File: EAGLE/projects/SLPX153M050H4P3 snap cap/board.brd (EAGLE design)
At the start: 139.7 x 64.4 mm, 6 parts

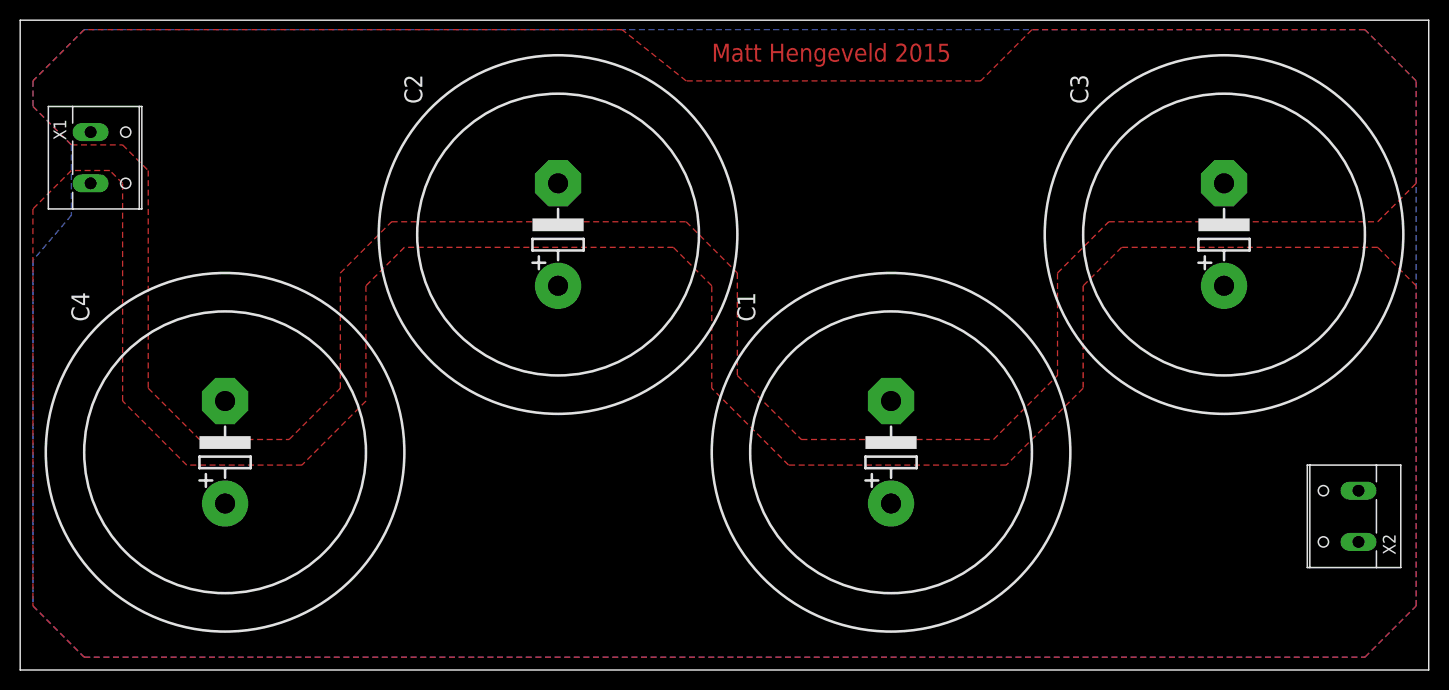
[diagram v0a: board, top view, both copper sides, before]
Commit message: a lot
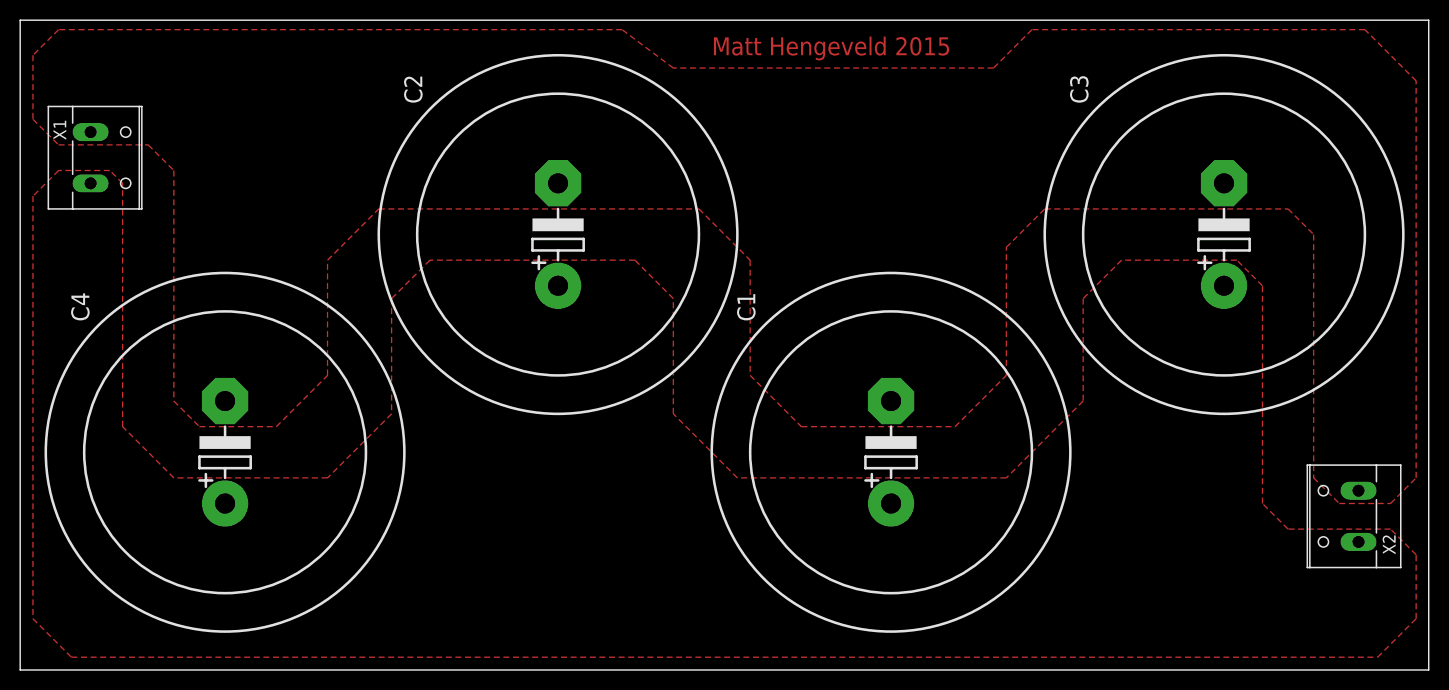
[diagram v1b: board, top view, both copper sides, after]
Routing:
- removed copper zone on layer 16, net GND
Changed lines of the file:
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@@
 <layer number="14" name="Route14" color="1" fill="6" visible="no" active="no"/>
 <layer number="15" name="Route15" color="4" fill="6" visible="no" active="no"/>
-<layer number="16" name="Bottom" color="1" fill="1" visible="yes" active="yes"/>
-<layer number="17" name="Pads" color="2" fill="1" visible="yes" active="yes"/>
-<layer number="18" name="Vias" color="2" fill="1" visible="yes" active="yes"/>
-<layer number="19" name="Unrouted" color="6" fill="1" visible="yes" active="yes"/>
-<layer number="20" name="Dimension" color="15" fill="1" visible="yes" active="yes"/>
-<layer number="21" name="tPlace" color="7" fill="1" visible="yes" active="yes"/>
-<layer number="22" name="bPlace" color="7" fill="1" visible="yes" active="yes"/>
-<layer number="23" name="tOrigins" color="15" fill="1" visible="yes" active="yes"/>
-<layer number="24" name="bOrigins" color="15" fill="1" visible="yes" active="yes"/>
-<layer number="25" name="tNames" color="7" fill="1" visible="yes" active="yes"/>
-<layer number="26" name="bNames" color="7" fill="1" visible="yes" active="yes"/>
-<layer number="27" name="tValues" color="7" fill="1" visible="yes" active="yes"/>
-<layer number="28" name="bValues" color="7" fill="1" visible="yes" active="yes"/>
+<layer number="16" name="Bottom" color="1" fill="1" visible="no" active="yes"/>
+<layer number="17" name="Pads" color="2" fill="1" visible="no" active="yes"/>
+<layer number="18" name="Vias" color="2" fill="1" visible="no" active="yes"/>
+<layer number="19" name="Unrouted" color="6" fill="1" visible="no" active="yes"/>
+<layer number="20" name="Dimension" color="15" fill="1" visible="no" active="yes"/>
+<layer number="21" name="tPlace" color="7" fill="1" visible="no" active="yes"/>
+<layer number="22" name="bPlace" color="7" fill="1" visible="no" active="yes"/>
+<layer number="23" name="tOrigins" color="15" fill="1" visible="no" active="yes"/>
+<layer number="24" name="bOrigins" color="15" fill="1" visible="no" active="yes"/>
+<layer number="25" name="tNames" color="7" fill="1" visible="no" active="yes"/>
+<layer number="26" name="bNames" color="7" fill="1" visible="no" active="yes"/>
+<layer number="27" name="tValues" color="7" fill="1" visible="no" active="yes"/>
+<layer number="28" name="bValues" color="7" fill="1" visible="no" active="yes"/>
 <layer number="29" name="tStop" color="7" fill="3" visible="no" active="yes"/>
 <layer number="30" name="bStop" color="7" fill="6" visible="no" active="yes"/>
@@
 <layer number="37" name="tTest" color="7" fill="1" visible="no" active="yes"/>
 <layer number="38" name="bTest" color="7" fill="1" visible="no" active="yes"/>
-<layer number="39" name="tKeepout" color="4" fill="11" visible="yes" active="yes"/>
-<layer number="40" name="bKeepout" color="1" fill="11" visible="yes" active="yes"/>
-<layer number="41" name="tRestrict" color="4" fill="10" visible="yes" active="yes"/>
-<layer number="42" name="bRestrict" color="1" fill="10" visible="yes" active="yes"/>
-<layer number="43" name="vRestrict" color="2" fill="10" visible="yes" active="yes"/>
+<layer number="39" name="tKeepout" color="4" fill="11" visible="no" active="yes"/>
+<layer number="40" name="bKeepout" color="1" fill="11" visible="no" active="yes"/>
+<layer number="41" name="tRestrict" color="4" fill="10" visible="no" active="yes"/>
+<layer number="42" name="bRestrict" color="1" fill="10" visible="no" active="yes"/>
+<layer number="43" name="vRestrict" color="2" fill="10" visible="no" active="yes"/>
 <layer number="44" name="Drills" color="7" fill="1" visible="no" active="yes"/>
 <layer number="45" name="Holes" color="7" fill="1" visible="no" active="yes"/>
 <layer number="46" name="Milling" color="3" fill="1" visible="no" active="yes"/>
 <layer number="47" name="Measures" color="7" fill="1" visible="no" active="yes"/>
-<layer number="48" name="Document" color="7" fill="1" visible="yes" active="yes"/>
-<layer number="49" name="Reference" color="7" fill="1" visible="yes" active="yes"/>
-<layer number="51" name="tDocu" color="7" fill="1" visible="yes" active="yes"/>
-<layer number="52" name="bDocu" color="7" fill="1" visible="yes" active="yes"/>
+<layer number="48" name="Document" color="7" fill="1" visible="no" active="yes"/>
+<layer number="49" name="Reference" color="7" fill="1" visible="no" active="yes"/>
+<layer number="51" name="tDocu" color="7" fill="1" visible="no" active="yes"/>
+<layer number="52" name="bDocu" color="7" fill="1" visible="no" active="yes"/>
 <layer number="91" name="Nets" color="2" fill="1" visible="no" active="no"/>
 <layer number="92" name="Busses" color="1" fill="1" visible="no" active="no"/>
@@
 <wire x1="139.68" y1="64.44" x2="0" y2="64.44" width="0" layer="20"/>
 <wire x1="0" y1="64.44" x2="0" y2="0" width="0" layer="20"/>
-<text x="68.58" y="60.325" size="1.778" layer="1">Matt Hengeveld 2015</text>
+<text x="68.58" y="60.96" size="1.778" layer="1">Matt Hengeveld 2015</text>
 </plain>
 <attributes>
@@
 <signals>
 <signal name="GND">
-<polygon width="0.4064" layer="16" isolate="2.54" thermals="no">
-<vertex x="133.35" y="63.5"/>
-<vertex x="6.35" y="63.5"/>
-<vertex x="1.27" y="58.42"/>
-<vertex x="1.27" y="55.88"/>
-<vertex x="5.08" y="52.07"/>
-<vertex x="5.08" y="45.085"/>
-<vertex x="1.27" y="40.64"/>
-<vertex x="1.27" y="6.35"/>
-<vertex x="6.35" y="1.27"/>
-<vertex x="133.35" y="1.27"/>
-<vertex x="138.43" y="6.35"/>
-<vertex x="138.43" y="58.42"/>
-</polygon>
-<polygon width="0.4064" layer="1" isolate="1.6764" thermals="no">
-<vertex x="6.35" y="63.5"/>
-<vertex x="1.27" y="58.42"/>
-<vertex x="1.27" y="55.88"/>
-<vertex x="5.08" y="52.07"/>
-<vertex x="10.16" y="52.07"/>
-<vertex x="12.7" y="49.53"/>
-<vertex x="12.7" y="27.94"/>
-<vertex x="17.78" y="22.86"/>
-<vertex x="26.67" y="22.86"/>
-<vertex x="31.75" y="27.94"/>
-<vertex x="31.75" y="39.37"/>
-<vertex x="36.83" y="44.45"/>
-<vertex x="66.04" y="44.45"/>
-<vertex x="71.12" y="39.37"/>
-<vertex x="71.12" y="29.21"/>
-<vertex x="77.47" y="22.86"/>
-<vertex x="96.52" y="22.86"/>
-<vertex x="102.87" y="29.21"/>
-<vertex x="102.87" y="39.37"/>
-<vertex x="107.95" y="44.45"/>
-<vertex x="134.62" y="44.45"/>
-<vertex x="138.43" y="48.26"/>
+<polygon width="0.4064" layer="1" isolate="0.6096" thermals="no">
+<vertex x="3.81" y="63.5"/>
+<vertex x="1.27" y="60.96"/>
+<vertex x="1.27" y="54.61"/>
+<vertex x="3.81" y="52.07"/>
+<vertex x="12.7" y="52.07"/>
+<vertex x="15.24" y="49.53"/>
+<vertex x="15.24" y="26.67"/>
+<vertex x="17.78" y="24.13"/>
+<vertex x="25.4" y="24.13"/>
+<vertex x="30.48" y="29.21"/>
+<vertex x="30.48" y="40.64"/>
+<vertex x="35.56" y="45.72"/>
+<vertex x="67.31" y="45.72"/>
+<vertex x="72.39" y="40.64"/>
+<vertex x="72.39" y="29.21"/>
+<vertex x="77.47" y="24.13"/>
+<vertex x="92.71" y="24.13"/>
+<vertex x="97.79" y="29.21"/>
+<vertex x="97.79" y="41.91"/>
+<vertex x="101.6" y="45.72"/>
+<vertex x="125.73" y="45.72"/>
+<vertex x="128.27" y="43.18"/>
+<vertex x="128.27" y="19.05"/>
+<vertex x="130.81" y="16.51"/>
+<vertex x="135.89" y="16.51"/>
+<vertex x="138.43" y="19.05"/>
 <vertex x="138.43" y="58.42"/>
 <vertex x="133.35" y="63.5"/>
 <vertex x="100.33" y="63.5"/>
-<vertex x="95.25" y="58.42"/>
-<vertex x="66.04" y="58.42"/>
+<vertex x="96.52" y="59.69"/>
+<vertex x="64.77" y="59.69"/>
 <vertex x="59.69" y="63.5"/>
 </polygon>
@@
 <signal name="V+">
 <polygon width="0.4064" layer="1" isolate="1.778" thermals="no">
-<vertex x="5.08" y="49.53"/>
-<vertex x="1.27" y="45.72"/>
-<vertex x="1.27" y="6.35"/>
-<vertex x="6.35" y="1.27"/>
-<vertex x="133.35" y="1.27"/>
-<vertex x="138.43" y="6.35"/>
-<vertex x="138.43" y="38.1"/>
-<vertex x="134.62" y="41.91"/>
-<vertex x="109.22" y="41.91"/>
-<vertex x="105.41" y="38.1"/>
-<vertex x="105.41" y="27.94"/>
-<vertex x="97.79" y="20.32"/>
-<vertex x="76.2" y="20.32"/>
-<vertex x="68.58" y="27.94"/>
-<vertex x="68.58" y="38.1"/>
-<vertex x="64.77" y="41.91"/>
-<vertex x="38.1" y="41.91"/>
-<vertex x="34.29" y="38.1"/>
-<vertex x="34.29" y="26.67"/>
-<vertex x="27.94" y="20.32"/>
-<vertex x="16.51" y="20.32"/>
-<vertex x="10.16" y="26.67"/>
+<vertex x="3.81" y="49.53"/>
+<vertex x="1.27" y="46.99"/>
+<vertex x="1.27" y="5.08"/>
+<vertex x="5.08" y="1.27"/>
+<vertex x="134.62" y="1.27"/>
+<vertex x="138.43" y="5.08"/>
+<vertex x="138.43" y="11.43"/>
+<vertex x="135.89" y="13.97"/>
+<vertex x="125.73" y="13.97"/>
+<vertex x="123.19" y="16.51"/>
+<vertex x="123.19" y="38.1"/>
+<vertex x="120.65" y="40.64"/>
+<vertex x="109.22" y="40.64"/>
+<vertex x="105.41" y="36.83"/>
+<vertex x="105.41" y="26.67"/>
+<vertex x="97.79" y="19.05"/>
+<vertex x="71.12" y="19.05"/>
+<vertex x="64.77" y="25.4"/>
+<vertex x="64.77" y="36.83"/>
+<vertex x="60.96" y="40.64"/>
+<vertex x="40.64" y="40.64"/>
+<vertex x="36.83" y="36.83"/>
+<vertex x="36.83" y="25.4"/>
+<vertex x="30.48" y="19.05"/>
+<vertex x="15.24" y="19.05"/>
+<vertex x="10.16" y="24.13"/>
 <vertex x="10.16" y="48.26"/>
 <vertex x="8.89" y="49.53"/>
